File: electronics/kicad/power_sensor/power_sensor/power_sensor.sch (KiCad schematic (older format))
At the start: 6 parts, among them P4 a

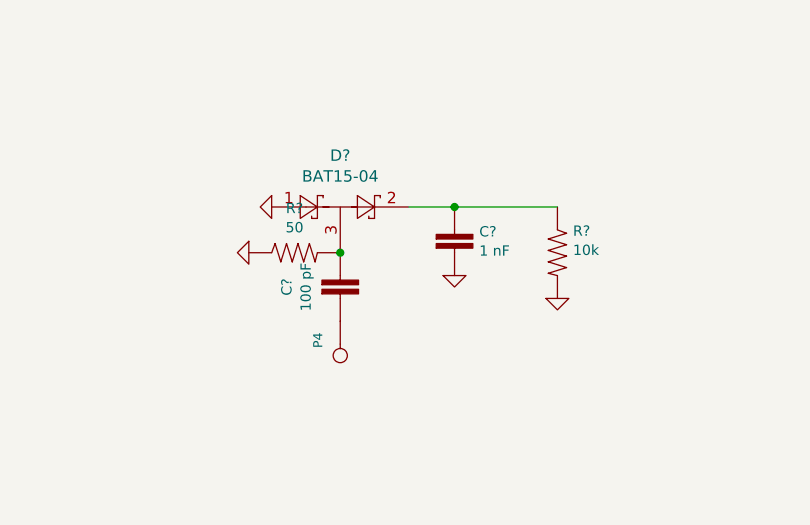
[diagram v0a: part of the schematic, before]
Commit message: Spectrum analyzer progress
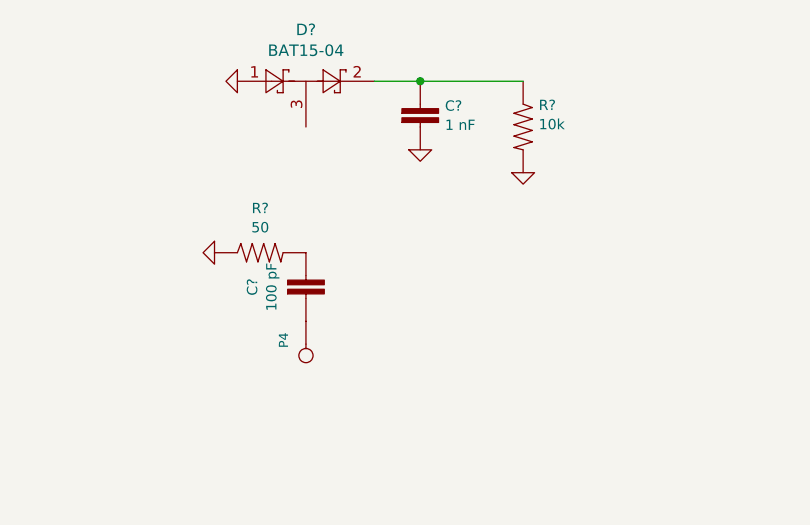
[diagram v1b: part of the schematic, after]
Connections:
- net at C?.1, R?.2: no longer D?.3
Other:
- moved on the sheet: C?, D?, P4, R?
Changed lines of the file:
@@
 L power:GND #PWR?
 U 1 1 5F014890
-P 5450 2300
-F 0 "#PWR?" H 5450 2300 30  0001 C CNN
-F 1 "GND" H 5450 2230 30  0001 C CNN
-F 2 "" H 5450 2300 50  0001 C CNN
-F 3 "" H 5450 2300 50  0001 C CNN
-	1    5450 2300
+P 5300 1750
+F 0 "#PWR?" H 5300 1750 30  0001 C CNN
+F 1 "GND" H 5300 1680 30  0001 C CNN
+F 2 "" H 5300 1750 50  0001 C CNN
+F 3 "" H 5300 1750 50  0001 C CNN
+	1    5300 1750
 	0    1    1    0
 $EndComp
@@
 L SparkFun-Capacitors:6PF-0402-50V-0.5% C?
 U 1 1 5F01536C
-P 6250 2500
-F 0 "C?" H 6358 2592 45  0000 L CNN
-F 1 "1 nF" H 6358 2508 45  0000 L CNN
-F 2 "0402" H 6250 2750 20  0001 C CNN
-F 3 "" H 6250 2500 50  0001 C CNN
-F 4 "" H 6358 2466 60  0000 L CNN "Field4"
-	1    6250 2500
+P 6100 1950
+F 0 "C?" H 6208 2042 45  0000 L CNN
+F 1 "1 nF" H 6208 1958 45  0000 L CNN
+F 2 "0402" H 6100 2200 20  0001 C CNN
+F 3 "" H 6100 1950 50  0001 C CNN
+F 4 "" H 6208 1916 60  0000 L CNN "Field4"
+	1    6100 1950
 	1    0    0    -1
 $EndComp
@@
 L power:GND #PWR?
 U 1 1 5F016B90
-P 6250 2600
-F 0 "#PWR?" H 6250 2600 30  0001 C CNN
-F 1 "GND" H 6250 2530 30  0001 C CNN
-F 2 "" H 6250 2600 50  0001 C CNN
-F 3 "" H 6250 2600 50  0001 C CNN
-	1    6250 2600
+P 6100 2050
+F 0 "#PWR?" H 6100 2050 30  0001 C CNN
+F 1 "GND" H 6100 1980 30  0001 C CNN
+F 2 "" H 6100 2050 50  0001 C CNN
+F 3 "" H 6100 2050 50  0001 C CNN
+	1    6100 2050
 	1    0    0    -1
 $EndComp
@@
 L conn:CONN_1 P4
 U 1 1 5EBA8EF1
-P 5750 2950
-F 0 "P4" H 5683 2853 40  0000 C CNN
-F 1 "a" H 5700 2990 30  0001 C CNN
-F 2 "TestPoint:TestPoint_Pad_1.5x1.5mm" H 5750 2950 50  0001 C CNN
-F 3 "" H 5750 2950 50  0001 C CNN
-	1    5750 2950
+P 5600 2950
+F 0 "P4" H 5533 2853 40  0000 C CNN
+F 1 "a" H 5550 2990 30  0001 C CNN
+F 2 "TestPoint:TestPoint_Pad_1.5x1.5mm" H 5600 2950 50  0001 C CNN
+F 3 "" H 5600 2950 50  0001 C CNN
+	1    5600 2950
 	0    1    1    0
 $EndComp
 Wire Wire Line
-	6250 2300 6050 2300
-Connection ~ 6250 2300
+	6100 1750 5900 1750
+Connection ~ 6100 1750
 $Comp
 L SparkFun-Resistors:RESISTOR0402 R?
 U 1 1 5F0217ED
-P 6700 2500
-F 0 "R?" V 6605 2568 45  0000 L CNN
-F 1 "10k" V 6689 2568 45  0000 L CNN
-F 2 "0402" H 6700 2650 20  0001 C CNN
-F 3 "" H 6700 2500 60  0001 C CNN
-F 4 " " V 6784 2568 60  0000 L CNN "Field4"
-	1    6700 2500
+P 6550 1950
+F 0 "R?" V 6455 2018 45  0000 L CNN
+F 1 "10k" V 6539 2018 45  0000 L CNN
+F 2 "0402" H 6550 2100 20  0001 C CNN
+F 3 "" H 6550 1950 60  0001 C CNN
+F 4 " " V 6634 2018 60  0000 L CNN "Field4"
+	1    6550 1950
 	0    1    1    0
 $EndComp
@@
 L power:GND #PWR?
 U 1 1 5F021FD0
-P 6700 2700
-F 0 "#PWR?" H 6700 2700 30  0001 C CNN
-F 1 "GND" H 6700 2630 30  0001 C CNN
-F 2 "" H 6700 2700 50  0001 C CNN
-F 3 "" H 6700 2700 50  0001 C CNN
-	1    6700 2700
+P 6550 2150
+F 0 "#PWR?" H 6550 2150 30  0001 C CNN
+F 1 "GND" H 6550 2080 30  0001 C CNN
+F 2 "" H 6550 2150 50  0001 C CNN
+F 3 "" H 6550 2150 50  0001 C CNN
+	1    6550 2150
 	1    0    0    -1
 $EndComp
 Wire Wire Line
-	6250 2300 6700 2300
+	6100 1750 6550 1750
 $Comp
 L SparkFun-Capacitors:6PF-0402-50V-0.5% C?
 U 1 1 5F022E92
-P 5750 2700
-F 0 "C?" V 5516 2750 45  0000 C CNN
-F 1 "100 pF" V 5600 2750 45  0000 C CNN
-F 2 "0402" H 5750 2950 20  0001 C CNN
-F 3 "" H 5750 2700 50  0001 C CNN
-F 4 "" H 5858 2666 60  0000 L CNN "Field4"
-	1    5750 2700
+P 5600 2700
+F 0 "C?" V 5366 2750 45  0000 C CNN
+F 1 "100 pF" V 5450 2750 45  0000 C CNN
+F 2 "0402" H 5600 2950 20  0001 C CNN
+F 3 "" H 5600 2700 50  0001 C CNN
+F 4 "" H 5708 2666 60  0000 L CNN "Field4"
+	1    5600 2700
 	1    0    0    -1
 $EndComp
@@
 L SparkFun-Resistors:0.3OHM-0805-1_8W-1% R?
 U 1 1 5F028E3F
-P 5550 2500
-F 0 "R?" H 5550 2694 45  0000 C CNN
-F 1 "50" H 5550 2610 45  0000 C CNN
-F 2 "0805" H 5550 2650 20  0001 C CNN
-F 3 "" H 5550 2500 60  0001 C CNN
-F 4 "" H 5550 2621 60  0000 C CNN "Field4"
-	1    5550 2500
+P 5400 2500
+F 0 "R?" H 5400 2694 45  0000 C CNN
+F 1 "50" H 5400 2610 45  0000 C CNN
+F 2 "0805" H 5400 2650 20  0001 C CNN
+F 3 "" H 5400 2500 60  0001 C CNN
+F 4 "" H 5400 2621 60  0000 C CNN "Field4"
+	1    5400 2500
 	1    0    0    -1
 $EndComp
@@
 L Diode:BAS40-04 D?
 U 1 1 5F013846
-P 5750 2400
-F 0 "D?" H 5750 2725 50  0000 C CNN
-F 1 "BAT15-04" H 5750 2634 50  0000 C CNN
-F 2 "Package_TO_SOT_SMD:SOT-23" H 5500 2700 50  0001 L CNN
-F 3 "http://www.vishay.com/docs/85701/bas40v.pdf" H 5630 2500 50  0001 C CNN
-	1    5750 2400
+P 5600 1850
+F 0 "D?" H 5600 2175 50  0000 C CNN
+F 1 "BAT15-04" H 5600 2084 50  0000 C CNN
+F 2 "Package_TO_SOT_SMD:SOT-23" H 5350 2150 50  0001 L CNN
+F 3 "http://www.vishay.com/docs/85701/bas40v.pdf" H 5480 1950 50  0001 C CNN
+	1    5600 1850
 	1    0    0    -1
 $EndComp
-Connection ~ 5750 2500
 $Comp
 L power:GND #PWR?
 U 1 1 5F0342F0
-P 5350 2500
-F 0 "#PWR?" H 5350 2500 30  0001 C CNN
-F 1 "GND" H 5350 2430 30  0001 C CNN
-F 2 "" H 5350 2500 50  0001 C CNN
-F 3 "" H 5350 2500 50  0001 C CNN
-	1    5350 2500
+P 5200 2500
+F 0 "#PWR?" H 5200 2500 30  0001 C CNN
+F 1 "GND" H 5200 2430 30  0001 C CNN
+F 2 "" H 5200 2500 50  0001 C CNN
+F 3 "" H 5200 2500 50  0001 C CNN
+	1    5200 2500
 	0    1    1    0
 $EndComp
